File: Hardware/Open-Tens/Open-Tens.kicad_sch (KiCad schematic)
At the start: 27 parts

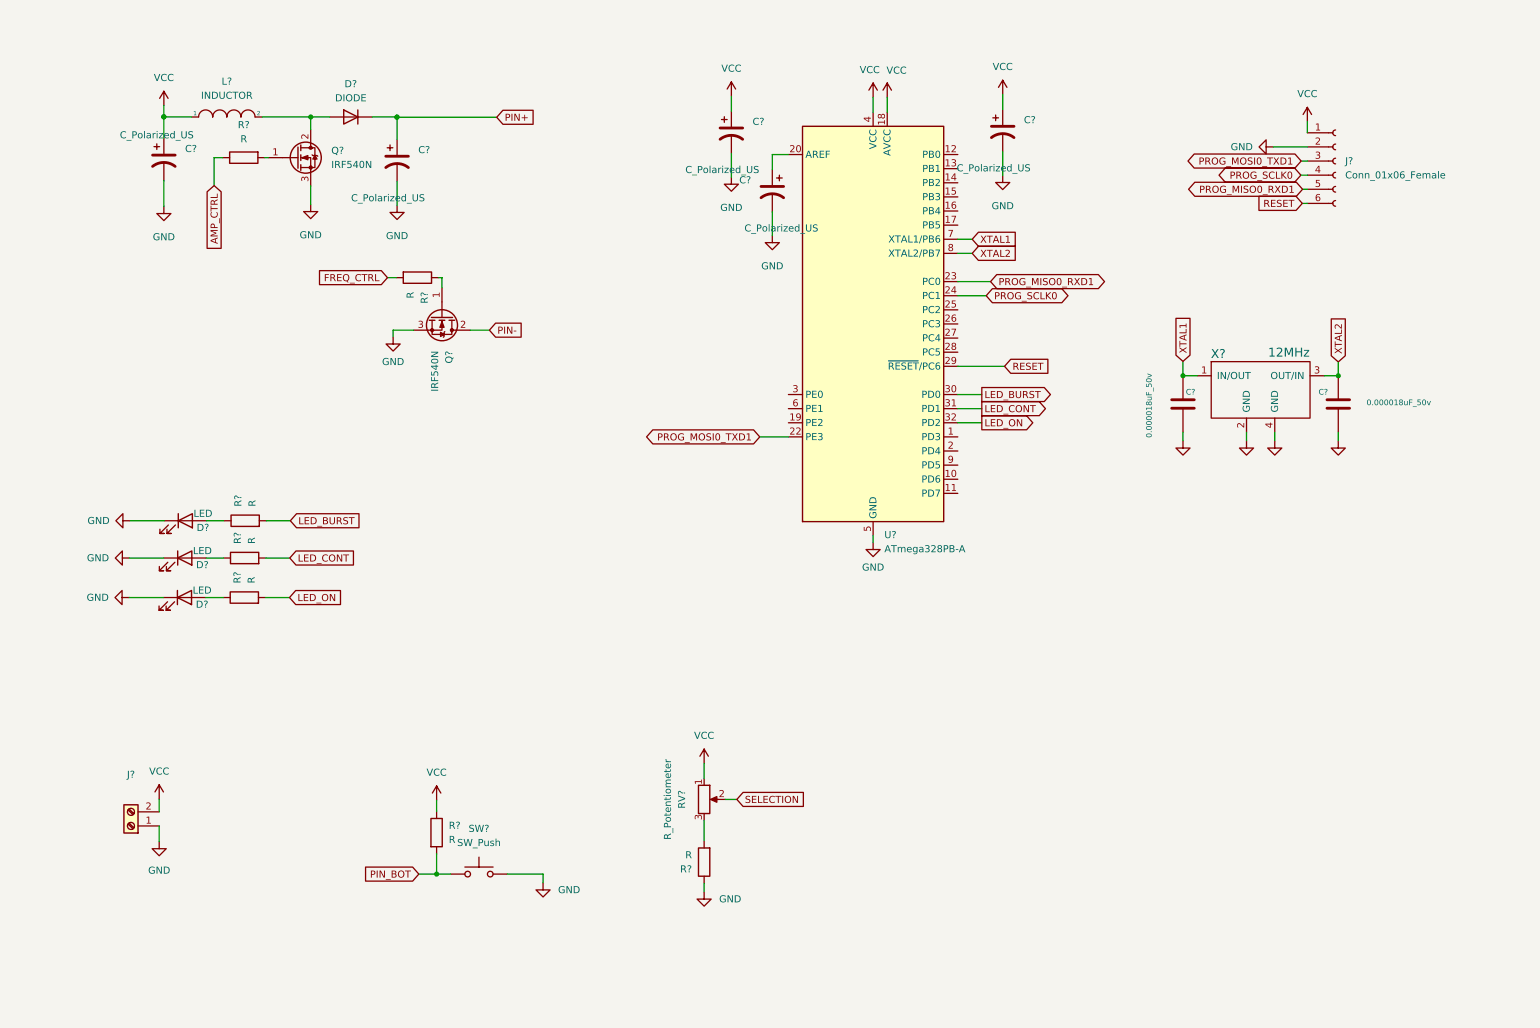
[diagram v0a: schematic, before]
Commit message: Separando o esquematico falta colocar valores
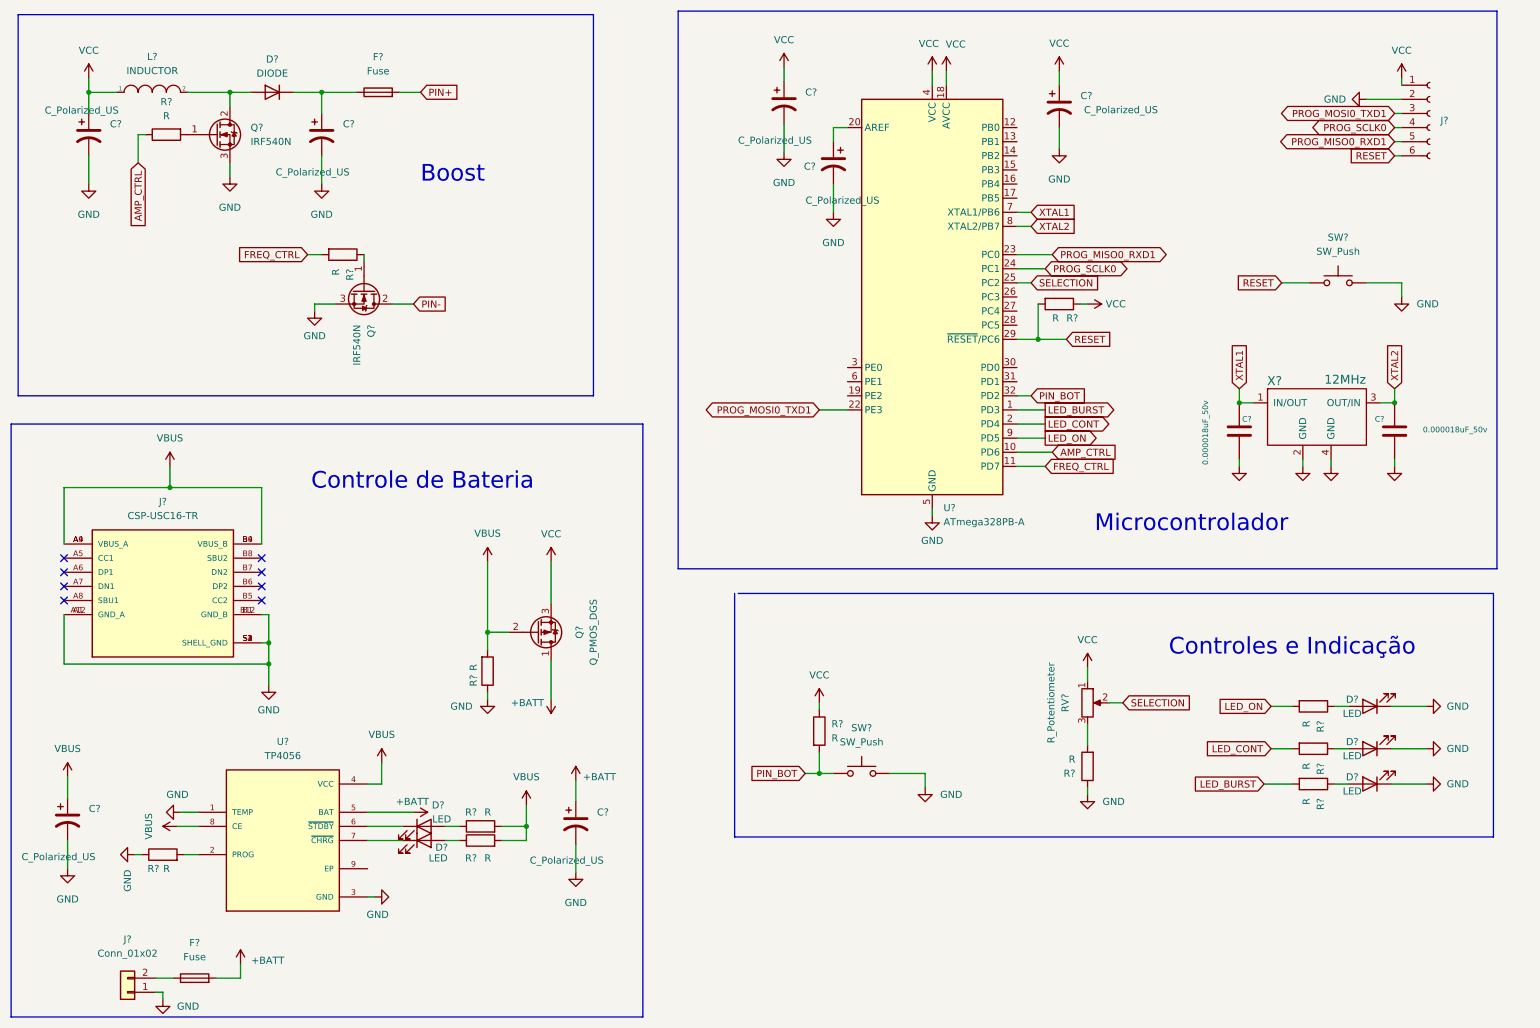
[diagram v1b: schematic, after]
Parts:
- removed J?: Screw_Terminal_01x02, symbol Connector:Screw_Terminal_01x02
- added C? (x2): C_Polarized_US, symbol Device:C_Polarized_US
- added D? (x2): LED, symbol Device:LED
- added F? (x2): Fuse, symbol Device:Fuse
- added J?: Conn_01x02, symbol Connector_Generic:Conn_01x02
- added J?: CSP-USC16-TR, VALCON_CSP-USC16-TR, symbol CSP-USC16-TR:CSP-USC16-TR
- added Q?: Q_PMOS_DGS, symbol Device:Q_PMOS_DGS
- added R? (x5): R, symbol Device:R
- added SW?: SW_Push, symbol Switch:SW_Push
- added U?: TP4056, SOP127P600X175-9N, symbol TP4056:TP4056
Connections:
- net AMP_CTRL: now also U?.10 (PD6)
- net FREQ_CTRL: now also U?.11 (PD7)
- net GND: now also C?.2, C?.2, J?.1 (Pin_1), J?.A1 (GND_A), J?.A12 (GND_A), J?.B1 (GND_B), J?.B12 (GND_B), J?.S1 (SHELL_GND), J?.S2 (SHELL_GND), J?.S3 (SHELL_GND), J?.S4 (SHELL_GND), R?.1, R?.1, SW?.2, U?.1 (TEMP), U?.3 (GND)
- net LED_BURST: now also U?.1 (PD3); no longer U?.30 (PD0)
- net LED_CONT: now also U?.2 (PD4); no longer U?.31 (PD1)
- net LED_ON: now also U?.9 (PD5); no longer U?.32 (PD2)
- net PIN+: now also F?.2
- net PIN_BOT: now also U?.32 (PD2)
- net RESET: now also R?.2, SW?.1
- net SELECTION: now also U?.25 (PC2)
- net VCC: now also C?.1, L?.1, Q?.3 (S), R?.1
- net at C?.1, D?.2 (K): now also F?.1
- new net: F?.1, J?.2 (Pin_2)
- new net: R?.2, U?.2 (PROG)
- new net: D?.1 (K), U?.6 (~{STDBY})
- new net: D?.1 (K), U?.7 (~{CHRG})
- new net: D?.2 (A), R?.1 (x2)
- new net +BATT: C?.1, F?.2, Q?.1 (D), U?.5 (BAT)
- new net VBUS: C?.1, J?.A4 (VBUS_A), J?.A9 (VBUS_A), J?.B4 (VBUS_B), J?.B9 (VBUS_B), Q?.2 (G), R?.2, R?.2, R?.2, U?.4 (VCC), U?.8 (CE)
- no-connect marks 0 -> 8
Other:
- note added: "Boost"
- note added: "Controle de Bateria"
- note added: "Controles e Indicação"
- note added: "Microcontrolador"
- moved on the sheet: C?, D?, J?, L?, Q?, R?, RV?, SW?, U?, X?
